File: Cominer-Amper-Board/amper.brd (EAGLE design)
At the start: 95 x 90 mm, 69 parts, among them IC1 OP-AMP, J2 AVR_SPI_PROG_5X2LOCK, J3 AUDIO_JACK_3.5MM_PTH, J4 AUDIO_JACK_3.5MM_PTH, J5 AUDIO_JACK_3.5MM_PTH, J6 AUDIO_JACK_3.5MM_PTH, J7 MOLEX-CPU-POWER, J8 POWER_JACKSLT, Q1 220mA/50V/3.5Ω, Q2 220mA/50V/3.5Ω, Q3 220mA/50V/3.5Ω, Q4 220mA/50V/3.5Ω, Q5 220mA/50V/3.5Ω, Q6 220mA/50V/3.5Ω, Q7 20V/2A, U1 ESP-07, U2 ATMEGA16U2, U3 LM1117-3.3v, U4 LM1117-5v, U5 ADS1015, U6 ADS1015, Y1 16MHz

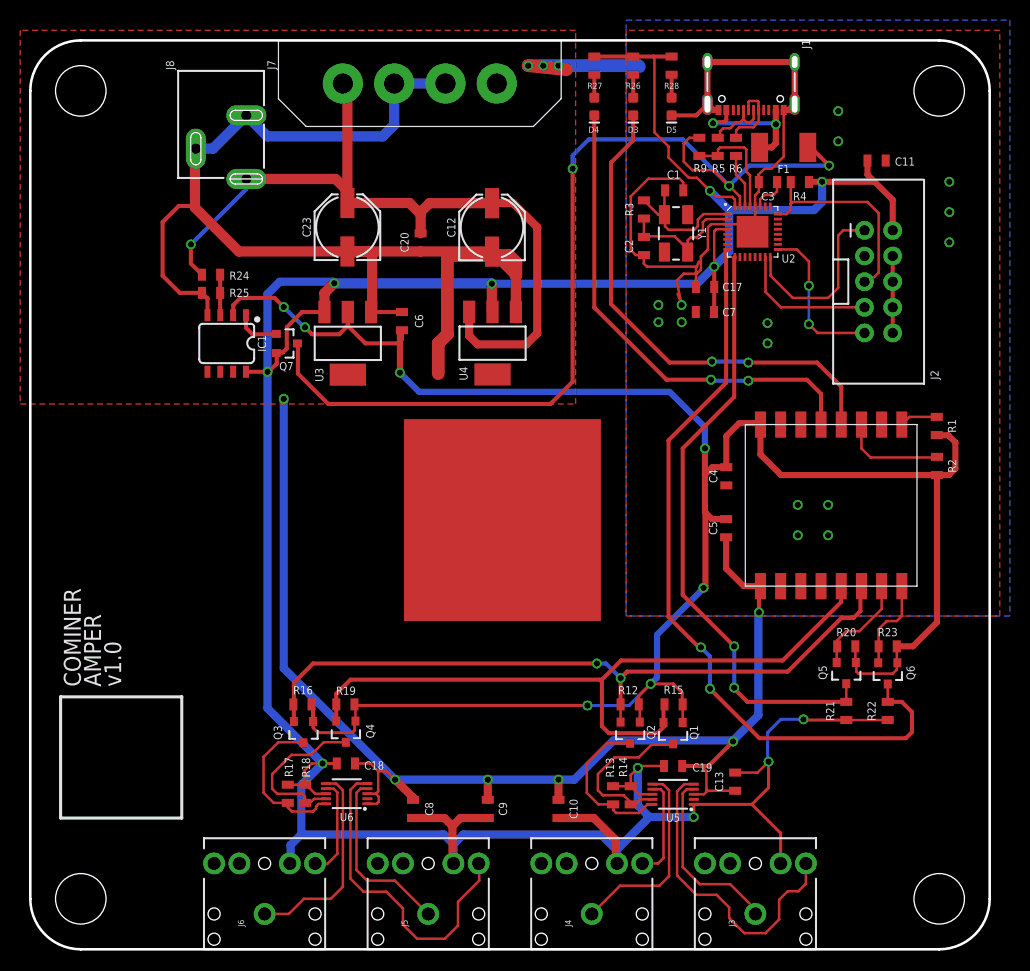
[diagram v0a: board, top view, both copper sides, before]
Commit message: amper board is ready
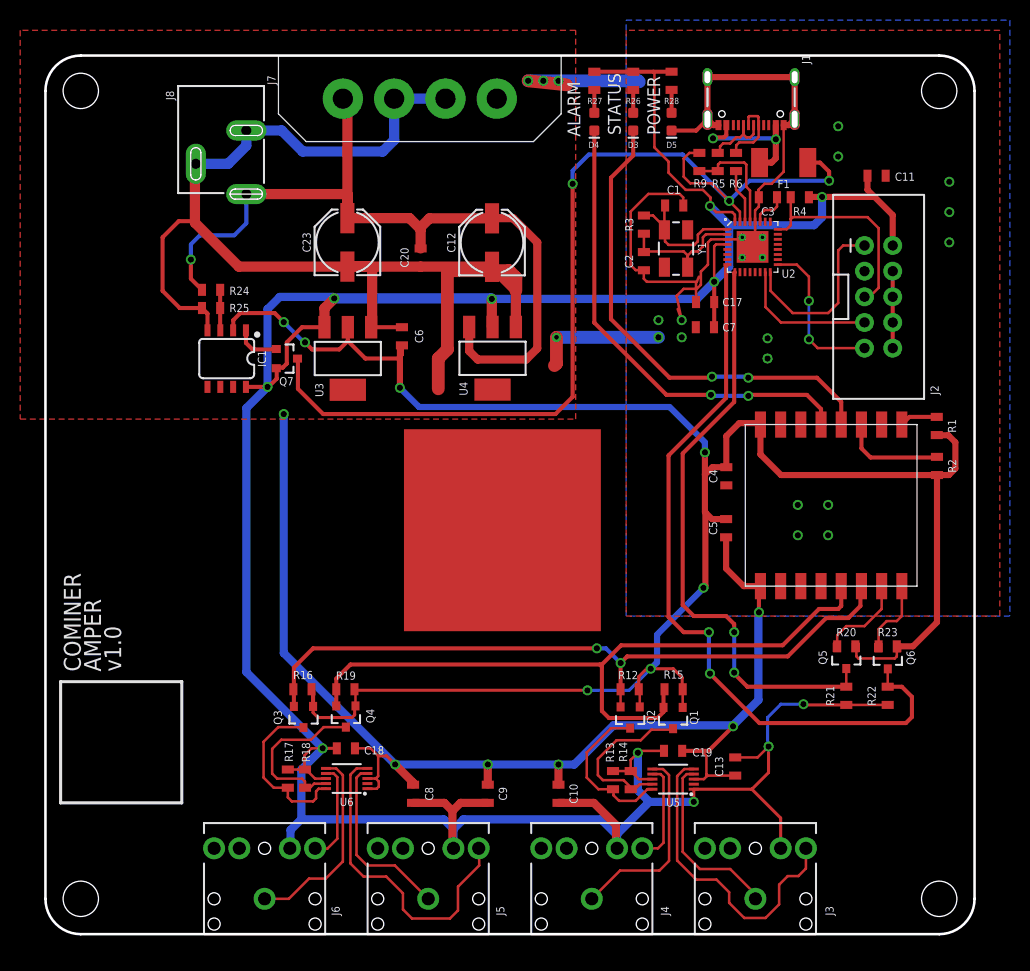
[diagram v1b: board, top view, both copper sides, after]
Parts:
- moved U5 1.50 mm to (63.6, 16.9)
- moved C1 1.50 mm to (63.8, 73.7)
- moved C10 1.50 mm to (52.3, 15.4)
- moved C11 1.50 mm to (83.8, 76.6)
- moved C12 1.50 mm to (45.7, 70.0)
- moved C13 1.50 mm to (69.8, 18.1)
- moved C17 1.50 mm to (66.8, 64.1)
- moved C18 1.50 mm to (31.2, 19.9)
- moved C19 1.50 mm to (63.6, 19.6)
- moved C2 1.50 mm to (60.8, 68.1)
- moved C20 1.50 mm to (38.6, 68.5)
- moved C23 1.50 mm to (31.4, 70.0)
- moved C3 1.50 mm to (73.0, 74.5)
- moved C6 1.50 mm to (36.8, 60.7)
- moved C7 1.50 mm to (66.8, 61.6)
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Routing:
- net GND: track 354.7 -> 364.1 mm, vias 24 -> 29
- net 3.3V: track 208.9 -> 203.3 mm
- net VIN: track 77.9 -> 80.6 mm
- net RX_AVR: track 76.6 -> 74.9 mm
- net TX_ESP: track 9.15 -> 7.65 mm
- net N$31: track 48.1 -> 46.6 mm
- net N$30: track 49.6 -> 48.1 mm
- net RX_ESP: track 10.2 -> 8.96 mm
- net TX_AVR: track 60.4 -> 59.3 mm
- net N$26: track 15.8 -> 16.8 mm
- net SCL_ADC: track 71.0 -> 70.1 mm
- net 5V: track 323.8 -> 323.1 mm
- net N$25: track 20.4 -> 19.8 mm
- net N$27: track 16.5 -> 17.1 mm
- net N$2: track 13.5 -> 14.0 mm
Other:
- board size 95 x 90 mm -> 92 x 87 mm
